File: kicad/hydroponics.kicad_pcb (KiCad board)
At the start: 2 copper layers, 9 parts, among them J1 ph-4502c, J2 TDS meter, J3 dht22, Q1 PN2222A, Q2 PN2222A, U1 Pico

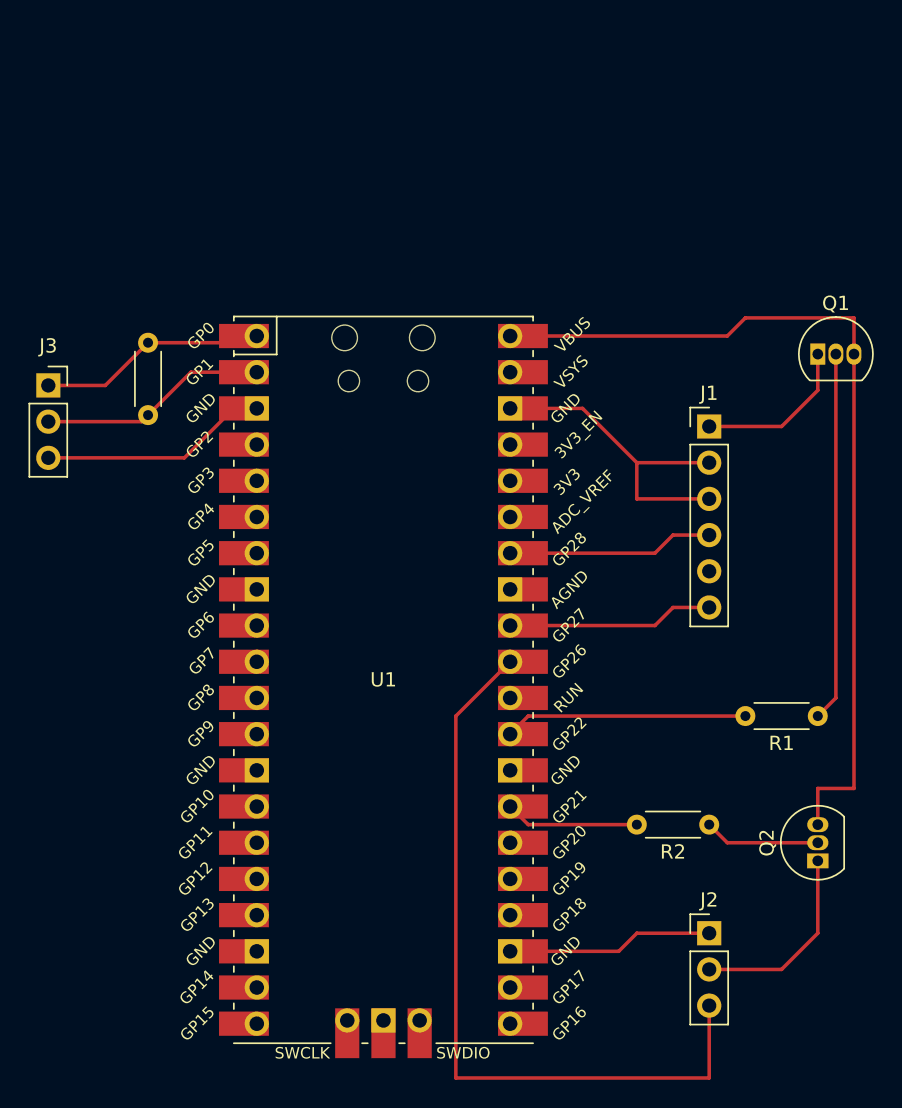
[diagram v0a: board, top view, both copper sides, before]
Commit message: chore: update kicad design
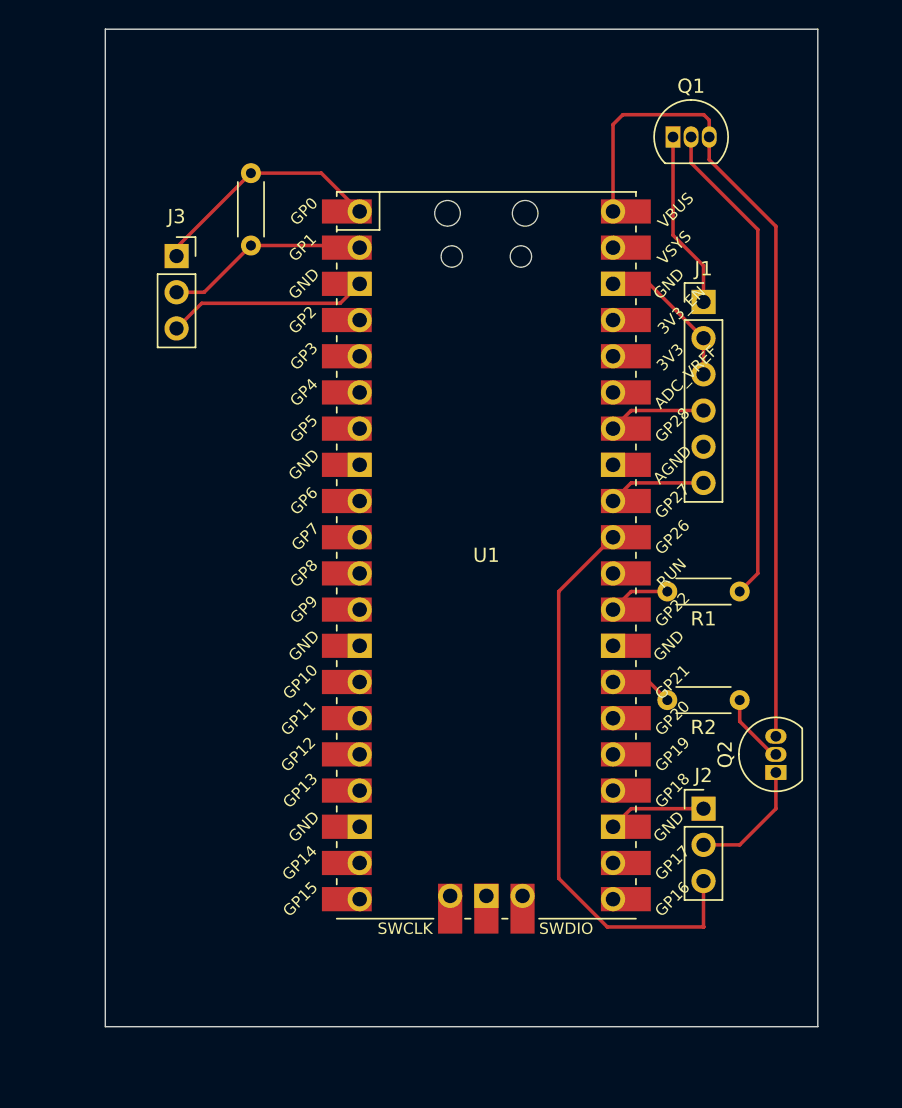
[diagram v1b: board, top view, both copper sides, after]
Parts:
- moved Q1 18.3 mm to (116.8, 35.6)
- moved R3 13.9 mm to (87.2, 38.1)
- moved J3 12.8 mm to (82.0, 43.9)
- moved U1 11.3 mm to (103.7, 64.9)
- moved R1 10.3 mm to (121.5, 67.5)
- moved R2 9.00 mm to (121.5, 75.1)
- moved J1 8.75 mm to (119.0, 47.1)
- moved J2 8.75 mm to (119.0, 82.7)
- moved Q2 6.86 mm to (124.1, 80.2)
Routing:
- net Net-(J2-A): track 53.6 -> 40.3 mm
- net Net-(U1-GPIO22): track 17.0 -> 4.34 mm
- net Net-(J1-GND-Pad2): track 23.2 -> 10.5 mm
- net Net-(Q1-B): track 25.9 -> 34.4 mm
- net Net-(J2--): track 14.5 -> 6.88 mm
- net Net-(J1-To): track 14.5 -> 6.88 mm
- net Net-(J1-Po): track 14.5 -> 6.88 mm
- net Net-(J2-+): track 13.8 -> 8.67 mm
- net Net-(U1-GPIO21): track 9.42 -> 4.34 mm
- net +5V: track 62.8 -> 58.5 mm
- net Net-(Q2-B): track 8.15 -> 4.99 mm
- net Net-(J3-O): track 16.1 -> 14.3 mm
- net +3.3V: track 15.4 -> 16.7 mm
- net Net-(J1-VCC): track 11.2 -> 12.5 mm
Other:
- board outline added: 50 x 70 mm
